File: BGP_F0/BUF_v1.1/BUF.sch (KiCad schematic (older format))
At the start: 36 parts, among them P1 CONN_01X02, P2 CONN_01X02, P3 CONN_01X03, P4 CONN_01X02, P5 Conn_01x06, P6 Conn_01x05, P7 CONN_01X02, Q1 2N5457, Q2 2N5457, U1 MC33178

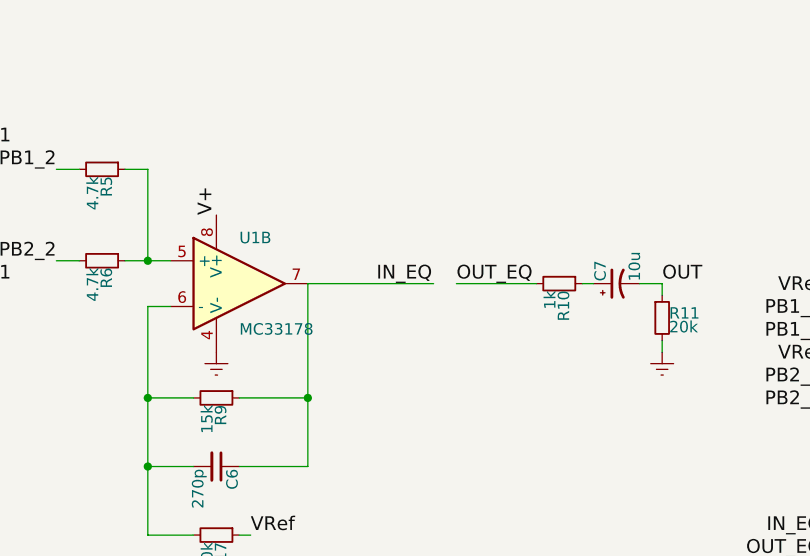
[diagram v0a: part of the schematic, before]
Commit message: Various
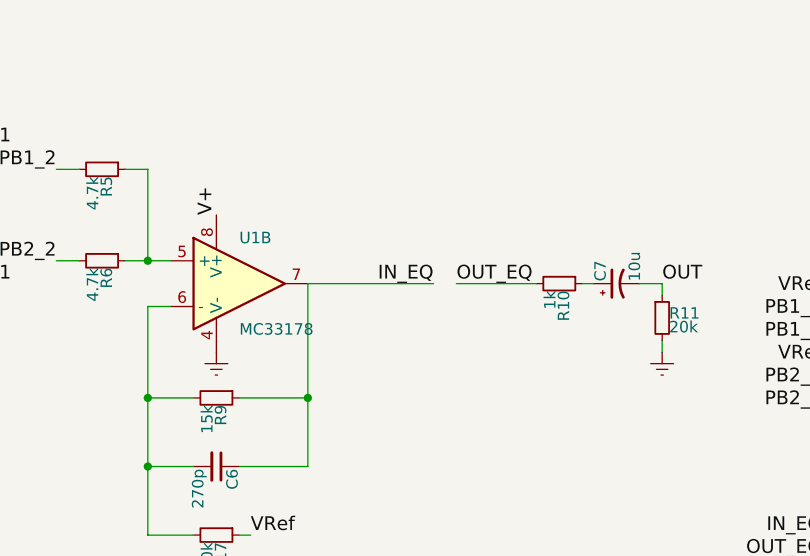
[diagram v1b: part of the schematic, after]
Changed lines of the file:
@@
 Text Label 7650 3300 0    60   ~ 0
 OUT
-Text Label 6400 3300 0    60   ~ 0
+Text Label 6650 3300 2    60   ~ 0
 IN_EQ
 Text Label 2400 3900 0    60   ~ 0

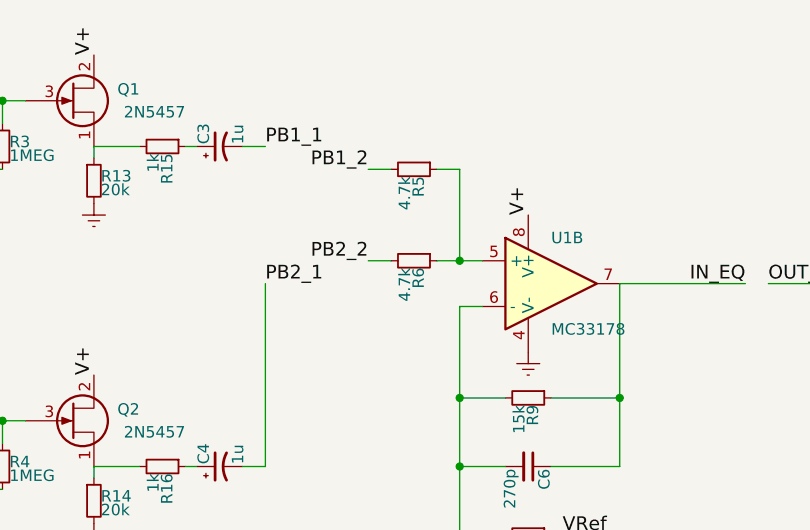
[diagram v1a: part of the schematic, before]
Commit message: Various
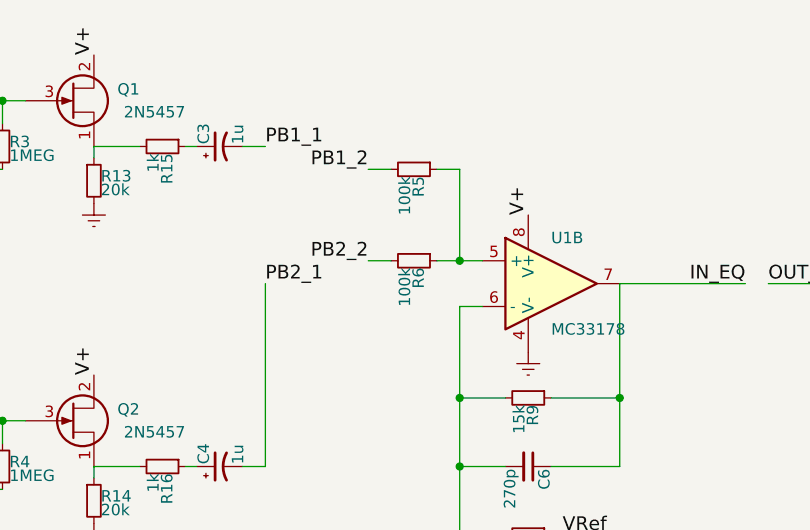
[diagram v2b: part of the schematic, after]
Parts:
- R5, R6: value 4.7k -> 100k
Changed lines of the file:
@@
 P 5200 2800
 F 0 "R5" H 5230 2820 50  0000 L CNN
-F 1 "4.7k" H 5230 2760 50  0000 L CNN
+F 1 "100k" H 5230 2760 50  0000 L CNN
 F 2 "Resistors_SMD:R_0603" H 5200 2800 50  0001 C CNN
 F 3 "" H 5200 2800 50  0000 C CNN
@@
 P 5200 3200
 F 0 "R6" H 5230 3220 50  0000 L CNN
-F 1 "4.7k" H 5230 3160 50  0000 L CNN
+F 1 "100k" H 5230 3160 50  0000 L CNN
 F 2 "Resistors_SMD:R_0603" H 5200 3200 50  0001 C CNN
 F 3 "" H 5200 3200 50  0000 C CNN
